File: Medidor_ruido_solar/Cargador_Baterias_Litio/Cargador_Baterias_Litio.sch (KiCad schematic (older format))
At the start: 9 parts, among them SW1 SW_DPDT_x2, U1 L7809

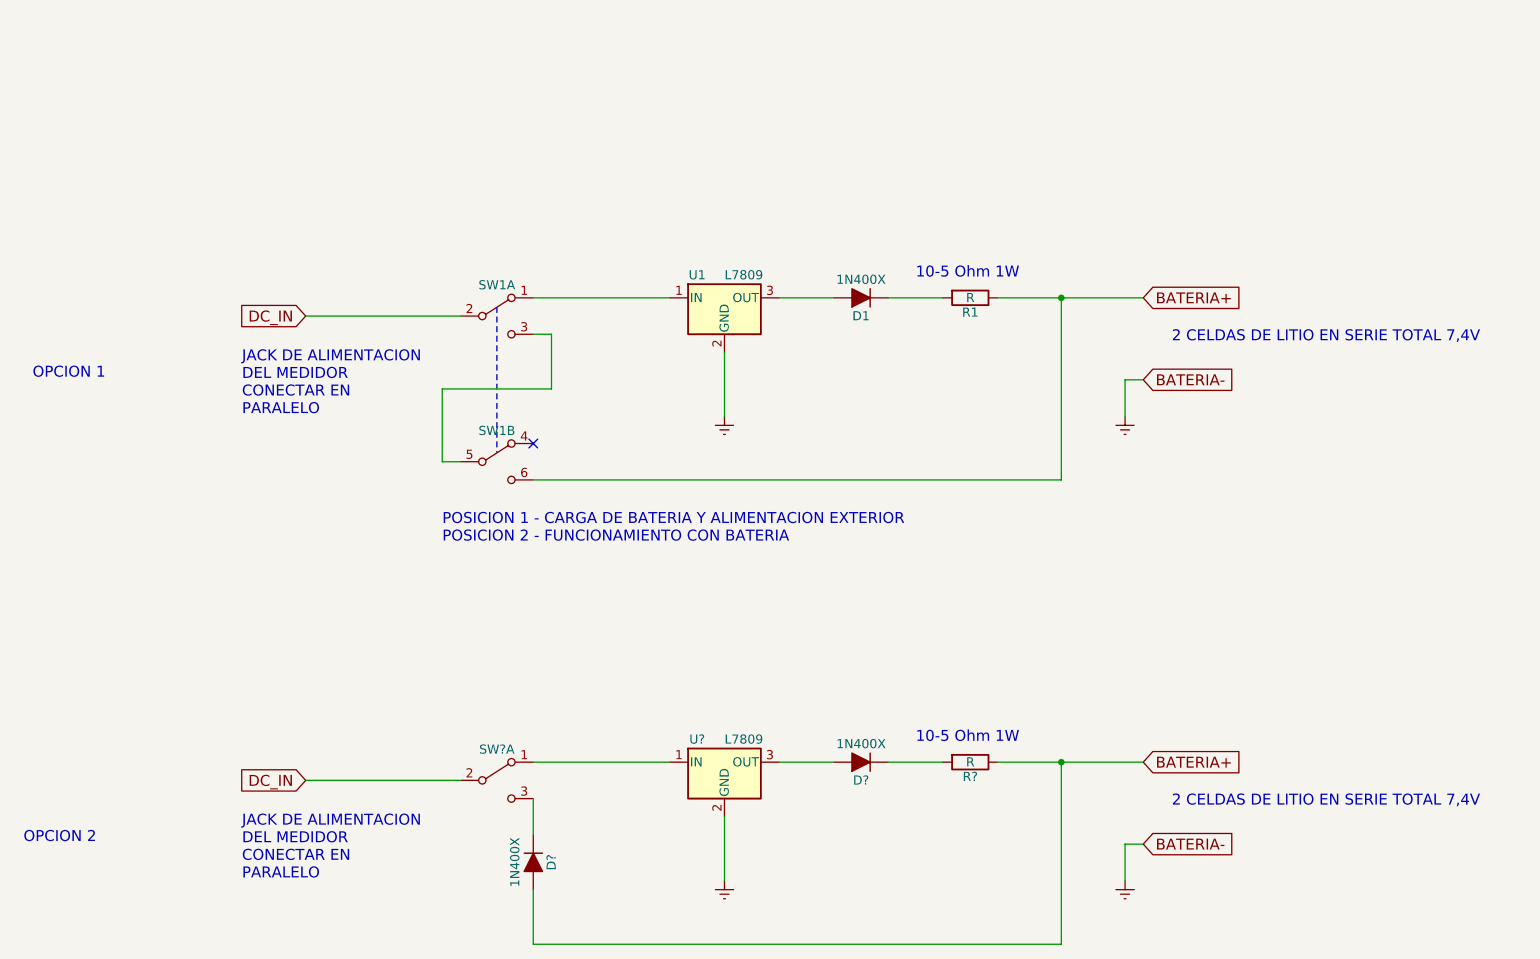
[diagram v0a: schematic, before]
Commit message: Medidor_Ruido_Solar
Cargador Balanceador
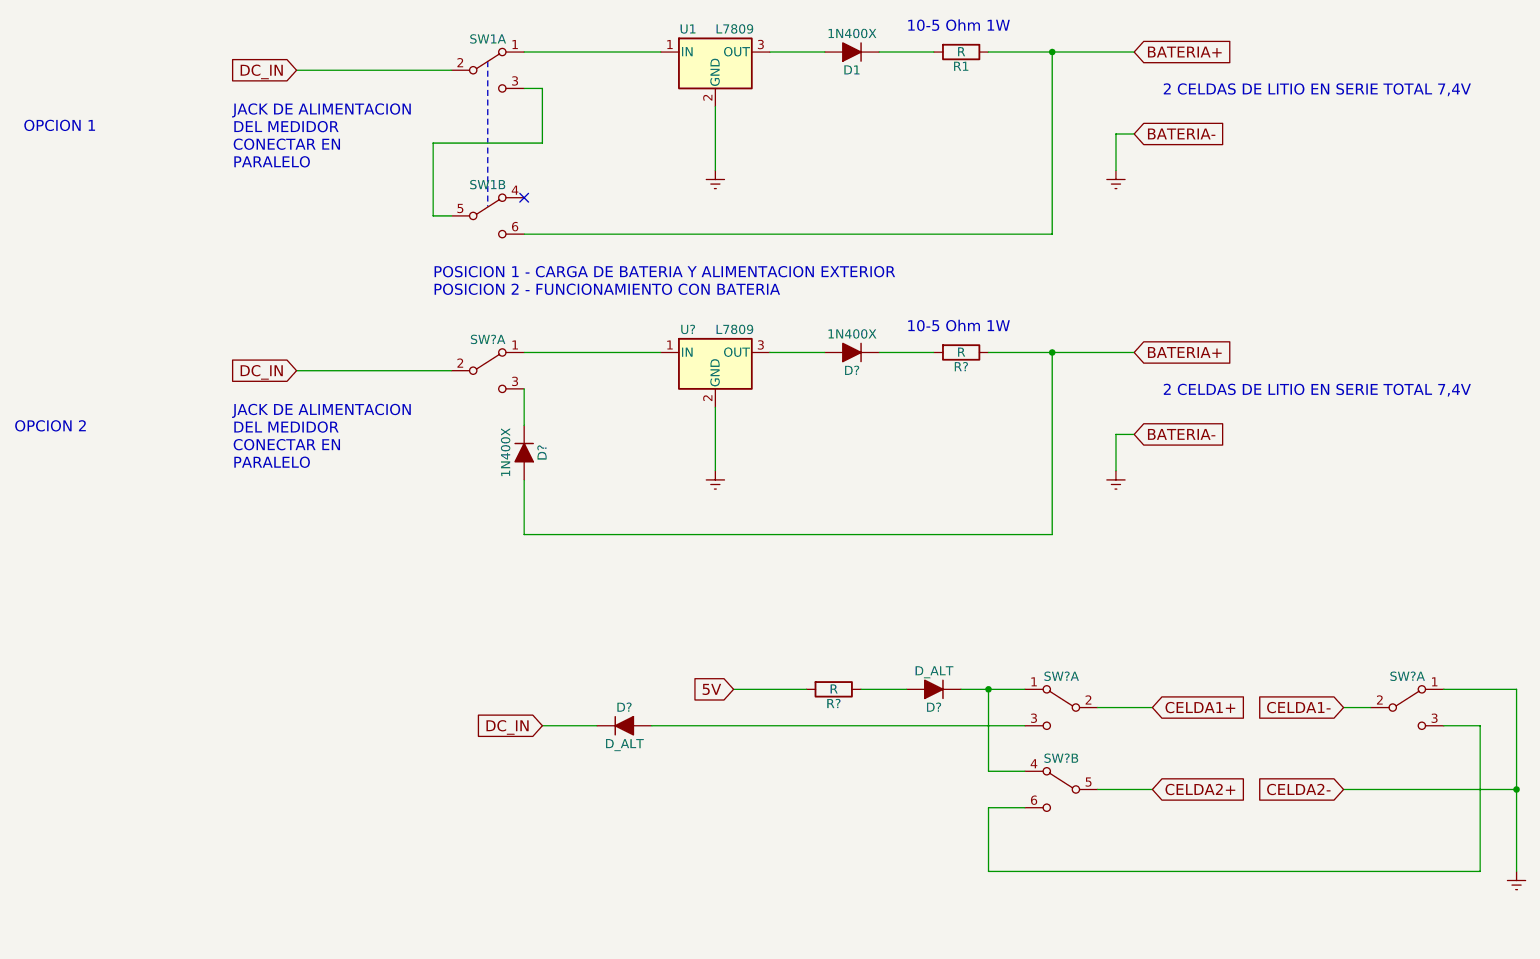
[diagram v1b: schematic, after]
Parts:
- added D? (x2): D_ALT, symbol D_ALT
- added R?: R, symbol R
- added SW? (x3): SW_DPDT_x2, symbol SW_DPDT_x2
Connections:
- net DC_IN: now also D?.1 (K)
- net GNDREF: now also SW?.1 (A)
- new net: D?.1 (K), SW?.1 (A), SW?.4 (A)
- new net: D?.2 (A), SW?.3 (C)
- new net: SW?.3 (C), SW?.6 (C)
- new net: D?.2 (A), R?.1
- new net 5V: R?.2
- new net CELDA1+: SW?.2 (B)
- new net CELDA1-: SW?.2 (B)
- new net CELDA2+: SW?.5 (B)
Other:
- moved on the sheet: D1, D?, R1, R?, SW1A, SW1B, SW?A, U1, U?

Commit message: Medidor_Ruido_Solar
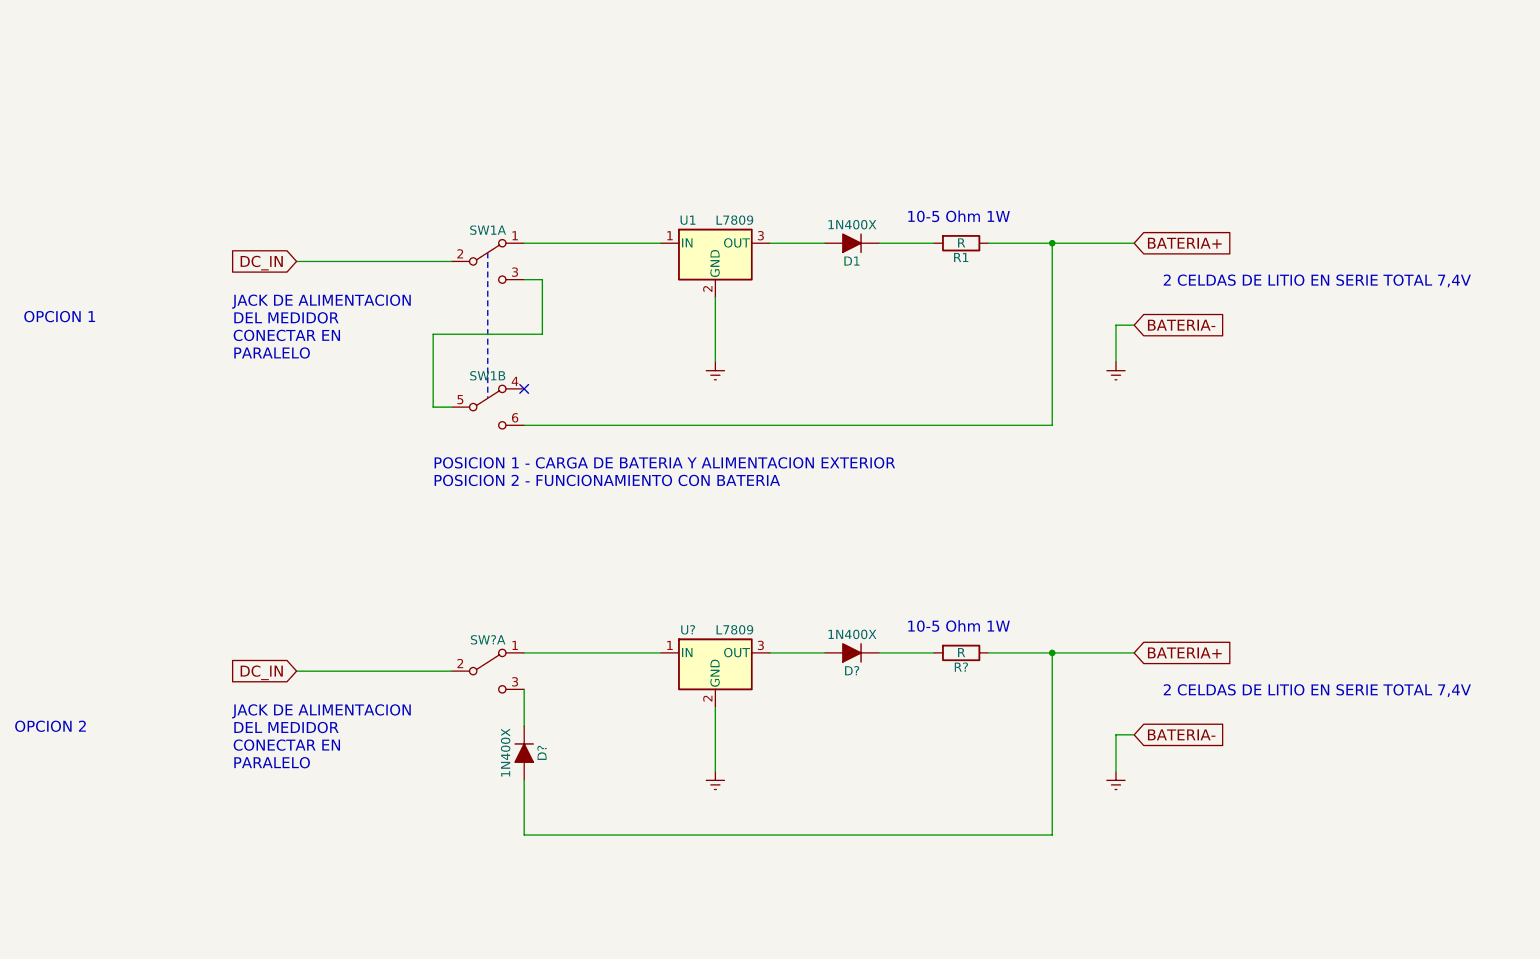
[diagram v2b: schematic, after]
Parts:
- removed D? (x2): D_ALT, symbol D_ALT
- removed R?: R, symbol R
- removed SW? (x3): SW_DPDT_x2, symbol SW_DPDT_x2
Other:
- moved on the sheet: D1, D?, R1, R?, SW1A, SW1B, SW?A, U1, U?
